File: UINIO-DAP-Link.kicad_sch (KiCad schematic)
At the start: 36 parts, among them J1 扩展板串口 & 电源输出, J2 扩展板 JTAG 输出, J3 JTAG_nTRST 跳线选择, J4 3.3V 跳线选择, J5 扩展板 SWD 输入, J6 DAPLink 固件下载接口, J7 JTAG/SWD 下载接口, U1 ME6211, U2 STM32F103C8T6, Y1 Crystal_GND24

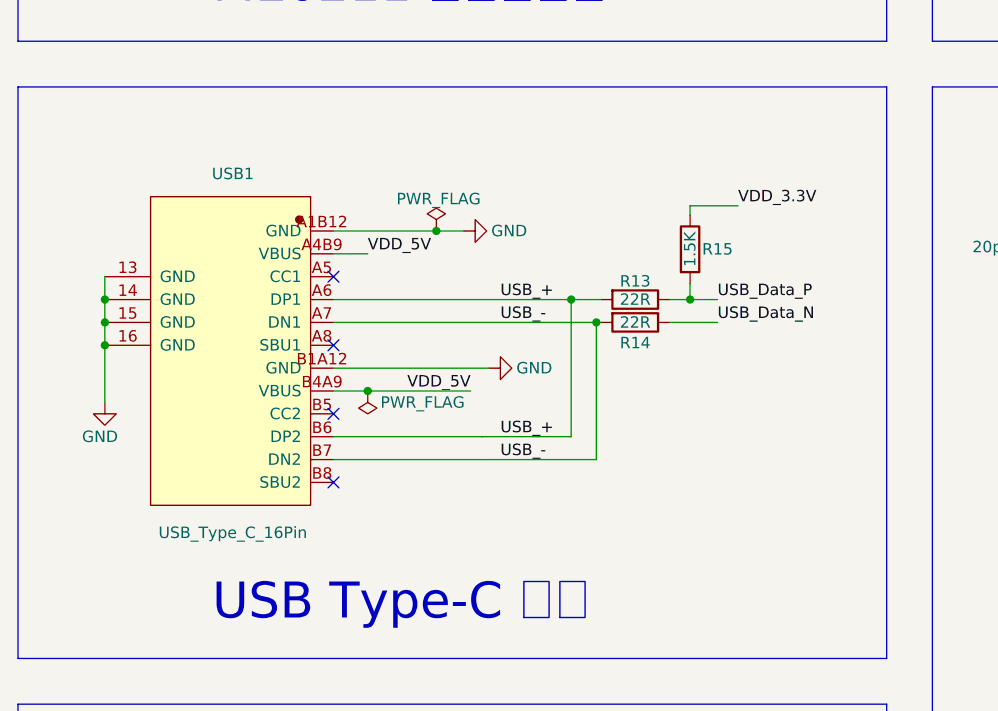
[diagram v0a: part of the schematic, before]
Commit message: Update PCB.
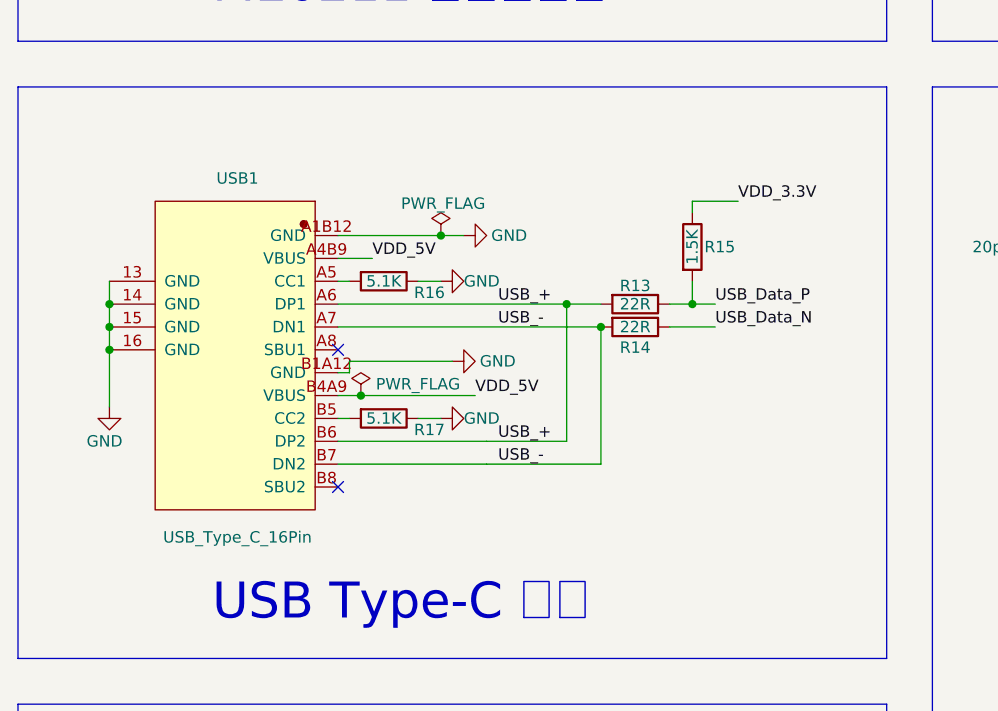
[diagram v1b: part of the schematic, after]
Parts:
- added R16, R17: 5.1K, Resistor_SMD:R_0603_1608Metric, symbol Device:R
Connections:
- net GND: now also R16.1, R17.1
- net at USB1.A5 (CC1): now also R16.2
- net at USB1.B5 (CC2): now also R17.2
- no-connect marks 28 -> 26
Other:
- moved on the sheet: R13, R14, USB1
